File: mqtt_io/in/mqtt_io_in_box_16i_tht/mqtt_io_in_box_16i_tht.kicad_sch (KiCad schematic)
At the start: 80 parts, among them J1 Conn_01x04_Pin, J2 Conn_01x04_Pin, U1 MCP23017_SP, U10 LTV-817, U11 LTV-817, U12 LTV-817, U13 LTV-817, U14 LTV-817, U15 LTV-817, U16 LTV-817, U17 LTV-817, U2 LTV-817, U3 LTV-817, U4 LTV-817, U5 LTV-817, U6 LTV-817, U7 LTV-817, U8 LTV-817, U9 LTV-817

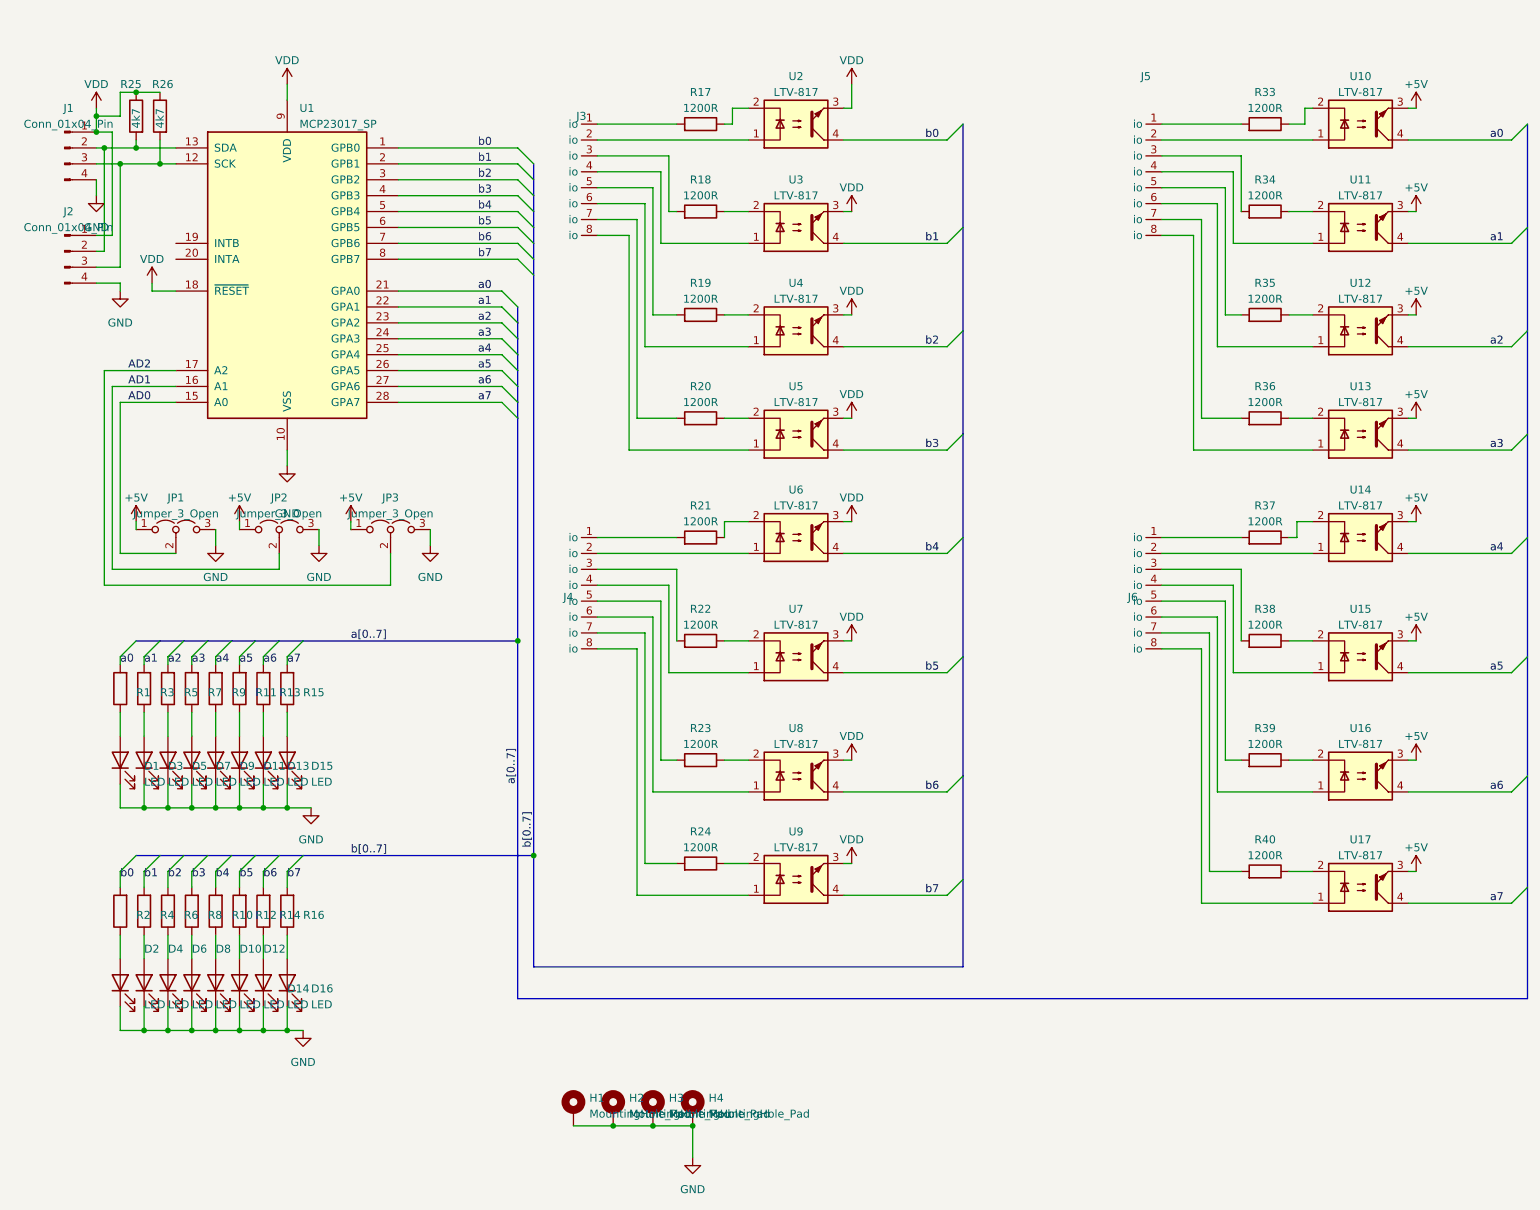
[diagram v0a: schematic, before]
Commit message: Add files via upload
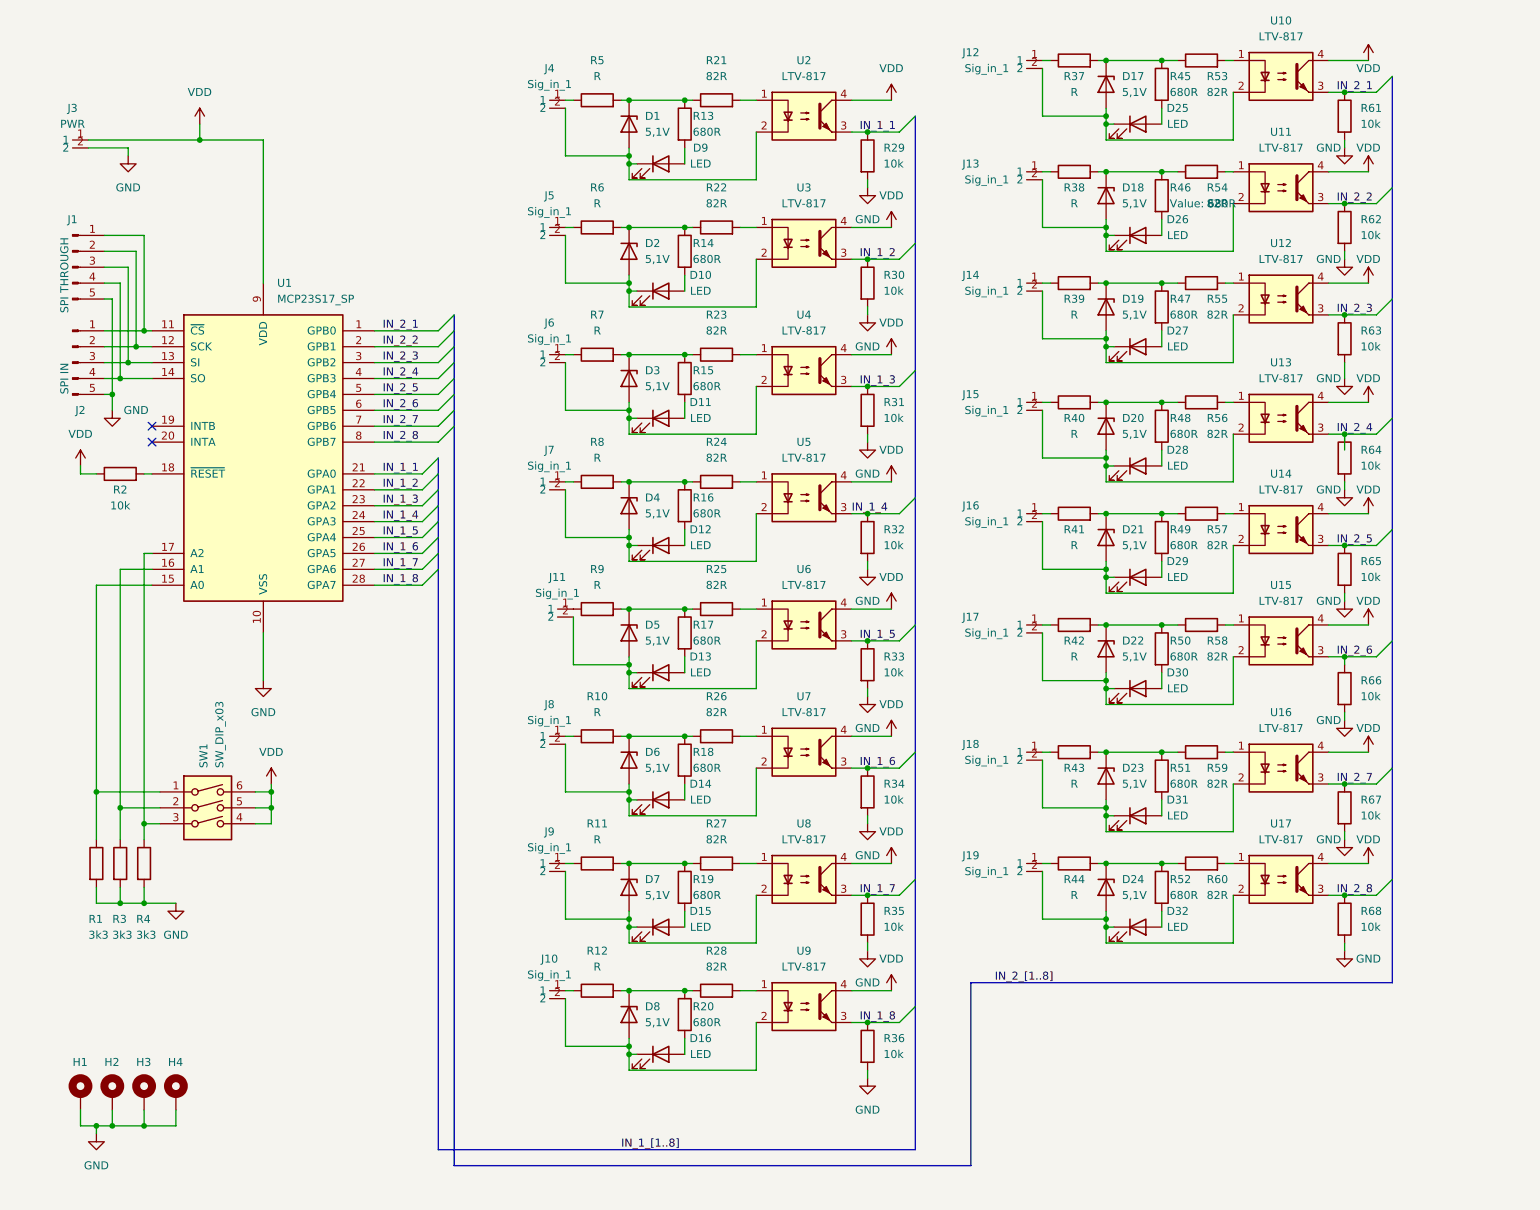
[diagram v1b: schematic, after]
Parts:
- removed D1, D2, D3, D4, D5, D6, D7, D8: LED, LED_THT:LED_D5.0mm, symbol Device:LED
- removed J1, J2: Conn_01x04_Pin, Connector_PinHeader_2.54mm:PinHeader_1x04_P2.54mm_Vertical, symbol Connector:Conn_01x04_Pin
- removed J3, J4, J5, J6: ~, parts_tma_1:AST041-08, symbol parts_tma_1:AST041-8
- removed JP1, JP2, JP3: Jumper_3_Open, Connector_PinHeader_2.54mm:PinHeader_1x03_P2.54mm_Vertical, symbol Jumper:Jumper_3_Open
- removed U1: MCP23017_SP, Package_DIP:DIP-28_W7.62mm, symbol Interface_Expansion:MCP23017_SP
- added D1, D17, D18, D19, D2, D20, D21, D22, D23, D24, D3, D4, D5, D6, D7, D8: 5,1V, Diode_THT:D_DO-41_SOD81_P10.16mm_Horizontal, symbol Device:D_Zener
- added D25, D26, D27, D28, D29, D30, D31, D32: LED, Diode_THT:D_DO-41_SOD81_P10.16mm_Horizontal, symbol Device:LED
- added J1: SPI THROUGH, Connector_PinHeader_2.54mm:PinHeader_1x05_P2.54mm_Vertical, symbol Connector:Conn_01x05_Pin
- added J10, J11, J12, J13, J14, J15, J16, J17, J18, J19, J4, J5, J6, J7, J8, J9: Sig_in_1, parts_tma_1:AST_041-2, symbol parts_tma_1:AST_041-2
- added J2: SPI IN, Connector_PinHeader_2.54mm:PinHeader_1x05_P2.54mm_Vertical, symbol Connector:Conn_01x05_Pin
- added J3: PWR, parts_tma_1:AST_041-2, symbol parts_tma_1:AST_041-2
- added R27, R28, R53, R54, R55, R56, R57, R58, R59, R60: 82R, Resistor_THT:R_Axial_DIN0204_L3.6mm_D1.6mm_P7.62mm_Horizontal, symbol Device:R
- added R29, R30, R31, R32, R61, R62, R63, R64, R65, R66, R67, R68: 10k, Resistor_THT:R_Axial_DIN0204_L3.6mm_D1.6mm_P7.62mm_Horizontal, symbol Device:R
- added R41, R42, R43, R44: R, Resistor_THT:R_Axial_DIN0204_L3.6mm_D1.6mm_P7.62mm_Horizontal, symbol Device:R
- added R45, R46, R47, R48, R49, R50, R51, R52: 680R, Resistor_THT:R_Axial_DIN0204_L3.6mm_D1.6mm_P7.62mm_Horizontal, symbol Device:R
- added SW1: SW_DIP_x03, Package_DIP:DIP-6_W7.62mm_LongPads, symbol Switch:SW_DIP_x03
- added U1: MCP23S17_SP, Package_DIP:DIP-28_W7.62mm, symbol Interface_Expansion:MCP23S17_SP
- R1, R3, R4: value 330R -> 3k3
- R10, R11, R12, R5, R6, R7, R8, R9: value 330R -> R
- R13, R14, R15, R16: value 330R -> 680R
- R17, R18, R19, R20: value 1200R -> 680R
- R2: value 330R -> 10k
- R21, R22, R23, R24: value 1200R -> 82R
- R25, R26: value 4k7 -> 82R
- R33, R34, R35, R36: value 1200R -> 10k
- R37, R38, R39, R40: value 1200R -> R
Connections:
- net GND: now also R1.2, R3.2, R33.2, R34.2, R35.2, R36.2, R4.2, J1.5 (Pin_5), J2.5 (Pin_5), J3.2, R29.2, R30.2, R31.2, R32.2, R61.2, R62.2, R63.2, R64.2, R65.2, R66.2, R67.2, R68.2, U1.10 (VSS); no longer D10.1 (K), D11.1 (K), D12.1 (K), D13.1 (K), D14.1 (K), D15.1 (K), D16.1 (K), D9.1 (K)
- net VDD: now also R2.1, U10.4, U11.4, U12.4, U13.4, U14.4, U15.4, U16.4, U17.4, U2.4, U3.4, U4.4, U5.4, U6.4, U7.4, U8.4, U9.4, J3.1, SW1.4, SW1.5, SW1.6, U1.9 (VDD); no longer R25.1, R26.1, U10.3, U11.3, U12.3, U13.3, U14.3, U15.3, U16.3, U17.3, U2.3, U3.3, U4.3, U5.3, U6.3, U7.3, U8.3, U9.3
- net at R26.2: now also U7.1
- net at R25.2: now also U6.1
- net at R21.2: now also U2.1
- net at R22.2: now also U3.1
- net at R23.2: now also U4.1
- net at U8.1: now also R27.2
- net at R24.2: now also U5.1
- net at U9.1: now also R28.2
- net at U8.2: now also D15.1 (K), D7.2 (A), J9.2; no longer R23.1
- net at U7.2: now also D14.1 (K), D6.2 (A), J8.2; no longer R22.1
- net at R12.1: now also J10.1; no longer D12.2 (A)
- net at U12.2: now also D19.2 (A), D27.1 (K), J14.2; no longer R35.1
- net at R13.1: now also R21.1, R5.2, D1.1 (K); no longer D13.2 (A)
- net at R3.1: now also SW1.2, U1.16 (A1)
- net at R10.1: now also J8.1; no longer D10.2 (A)
- net at U9.2: now also D16.1 (K), D8.2 (A), J10.2; no longer R24.1
- net at R16.1: now also R24.1, R8.2, D4.1 (K); no longer D16.2 (A)
- net at R8.1: now also J7.1
- net at R9.1: now also J11.1; no longer D9.2 (A)
- net at U15.1: now also R58.2
- net at U15.2: now also D22.2 (A), D30.1 (K), J17.2; no longer R38.1
- net at R19.1: now also R11.2, D7.1 (K), R27.1; no longer U4.2
- net at R19.2: now also D15.2 (A)
- net at R18.1: now also R10.2, R26.1, D6.1 (K); no longer U3.2
- net at R18.2: now also D14.2 (A)
- net at R14.1: now also R22.1, R6.2, D2.1 (K); no longer D14.2 (A)
- net at R15.1: now also R23.1, R7.2, D3.1 (K); no longer D15.2 (A)
- net at R1.1: now also SW1.1, U1.15 (A0)
- net at U6.2: now also D13.1 (K), D5.2 (A), J11.2; no longer R21.1
- net at U14.1: now also R57.2
- net at U14.2: now also D21.2 (A), D29.1 (K), J16.2; no longer R37.1
- net at D11.2 (A): now also R15.2; no longer R11.1
- net at U2.2: now also D9.1 (K), D1.2 (A), J4.2; no longer R17.1
- net at U12.1: now also R55.2
- net at U16.2: now also D23.2 (A), D31.1 (K), J18.2; no longer R39.1
- net at R39.2: now also D19.1 (K), R47.1, R55.1
- net at R17.2: now also D13.2 (A)
- net at R20.2: now also D16.2 (A)
- net at U13.2: now also D20.2 (A), D28.1 (K), J15.2; no longer R36.1
- net at U16.1: now also R59.2
- net at R4.1: now also SW1.3, U1.17 (A2)
- net at U10.2: now also D17.2 (A), D25.1 (K), J12.2; no longer R33.1
- net at R5.1: now also J4.1
- net at R20.1: now also R12.2, D8.1 (K), R28.1; no longer U5.2
- net at U10.1: now also R53.2
- net at U11.1: now also R54.2
- net at U13.1: now also R56.2
- net at R7.1: now also J6.1
- net at R6.1: now also J5.1
- net at R37.2: now also D17.1 (K), R45.1, R53.1
- net at U17.2: now also D24.2 (A), D32.1 (K), J19.2; no longer R40.1
- net at R40.2: now also D20.1 (K), R48.1, R56.1
- net at U11.2: now also D18.2 (A), D26.1 (K), J13.2; no longer R34.1
- net at R38.2: now also D18.1 (K), R46.1, R54.1
- net at U17.1: now also R60.2
- removed net a0: R1.2, U10.4
- removed net a1: R3.2, U11.4
- removed net a2: R5.2, U12.4
- removed net a3: R7.2, U13.4
- net a4: no longer names the net of R9.2
- net a4: now also R17.1, R25.1, D5.1 (K); no longer U14.4
- removed net a5: R11.2, U15.4
- net a6: no longer names the net of R13.2
- net a6: now also D9.2 (A); no longer U16.4
- removed net a7: R15.2, U17.4
- net b0: no longer names the net of R2.2
- net b0: now also U1.18 (~{RESET}); no longer U2.4
- removed net b1: R4.2, U3.4
- removed net b2: R6.2, U4.4
- removed net b3: R8.2, U5.4
- removed net b4: R10.2, U6.4
- removed net b5: R12.2, U7.4
- net b6: no longer names the net of R14.2
- net b6: now also D10.2 (A); no longer U8.4
- net b7: no longer names the net of R16.2
- net b7: now also D12.2 (A); no longer U9.4
- new net: D21.1 (K), R41.2, R49.1, R57.1
- new net: J19.1, R44.1
- new net: D22.1 (K), R42.2, R50.1, R58.1
- new net: D30.2 (A), R50.2
- new net: J16.1, R41.1
- new net: D27.2 (A), R47.2
- new net: D23.1 (K), R43.2, R51.1, R59.1
- new net: J12.1, R37.1
- new net: D29.2 (A), R49.2
- new net: J13.1, R38.1
- new net: D24.1 (K), R44.2, R52.1, R60.1
- new net: D25.2 (A), R45.2
- new net: D26.2 (A), R46.2
- new net: D11.1 (K), D3.2 (A), J6.2, U4.2
- new net: D12.1 (K), D4.2 (A), J7.2, U5.2
- new net: D10.1 (K), D2.2 (A), J5.2, U3.2
- new net: J15.1, R40.1
- new net: J17.1, R42.1
- new net: J18.1, R43.1
- new net: D31.2 (A), R51.2
- new net: D32.2 (A), R52.2
- new net: J1.1 (Pin_1), J2.1 (Pin_1), U1.11 (~{CS})
- new net: J1.2 (Pin_2), J2.2 (Pin_2), U1.12 (SCK)
- new net: J1.3 (Pin_3), J2.3 (Pin_3), U1.13 (SI)
- new net: J1.4 (Pin_4), J2.4 (Pin_4), U1.14 (SO)
- new net: J9.1, R11.1
- new net: J14.1, R39.1
- new net: D28.2 (A), R48.2
- new net IN_1_1: R29.1, U1.21 (GPA0), U2.3
- new net IN_1_2: R30.1, U1.22 (GPA1), U3.3
- new net IN_1_3: R31.1, U1.23 (GPA2), U4.3
- new net IN_1_4: R32.1, U1.24 (GPA3), U5.3
- new net IN_1_5: R33.1, U1.25 (GPA4), U6.3
- new net IN_1_6: R34.1, U1.26 (GPA5), U7.3
- new net IN_1_7: R35.1, U1.27 (GPA6), U8.3
- new net IN_1_8: R36.1, U1.28 (GPA7), U9.3
- new net IN_2_1: R61.1, U1.1 (GPB0), U10.3
- new net IN_2_2: R62.1, U1.2 (GPB1), U11.3
- new net IN_2_3: R63.1, U1.3 (GPB2), U12.3
- new net IN_2_4: R64.1, U1.4 (GPB3), U13.3
- new net IN_2_5: R65.1, U1.5 (GPB4), U14.3
- new net IN_2_6: R66.1, U1.6 (GPB5), U15.3
- new net IN_2_7: R67.1, U1.7 (GPB6), U16.3
- new net IN_2_8: R68.1, U1.8 (GPB7), U17.3
- no-connect marks 0 -> 2
